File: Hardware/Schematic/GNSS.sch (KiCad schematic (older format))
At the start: 1 part

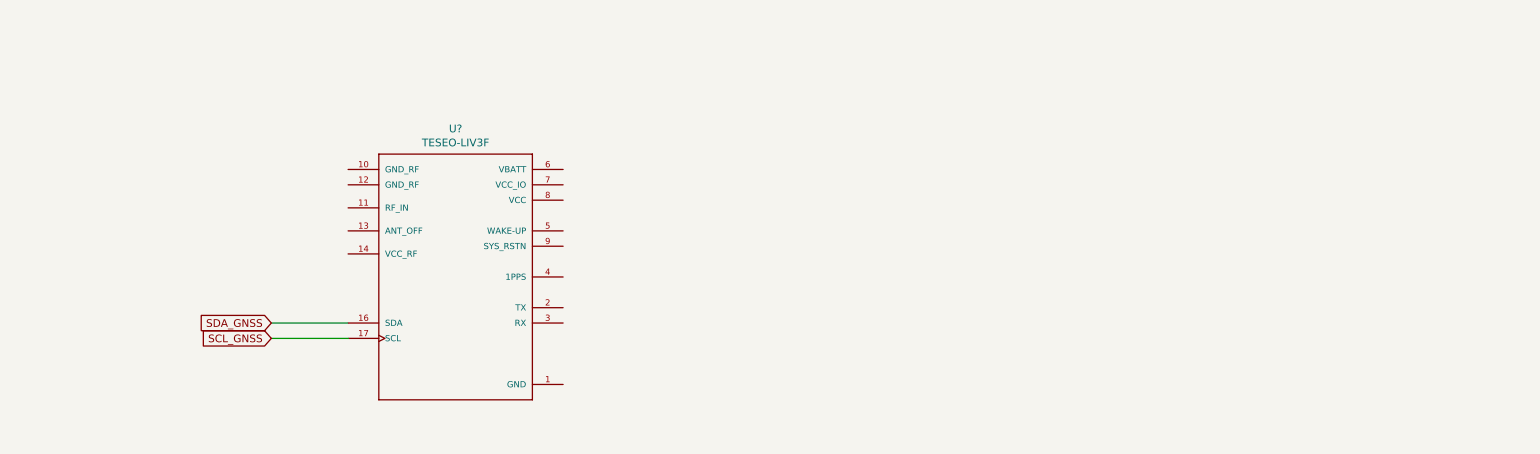
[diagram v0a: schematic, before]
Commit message: Add files via upload
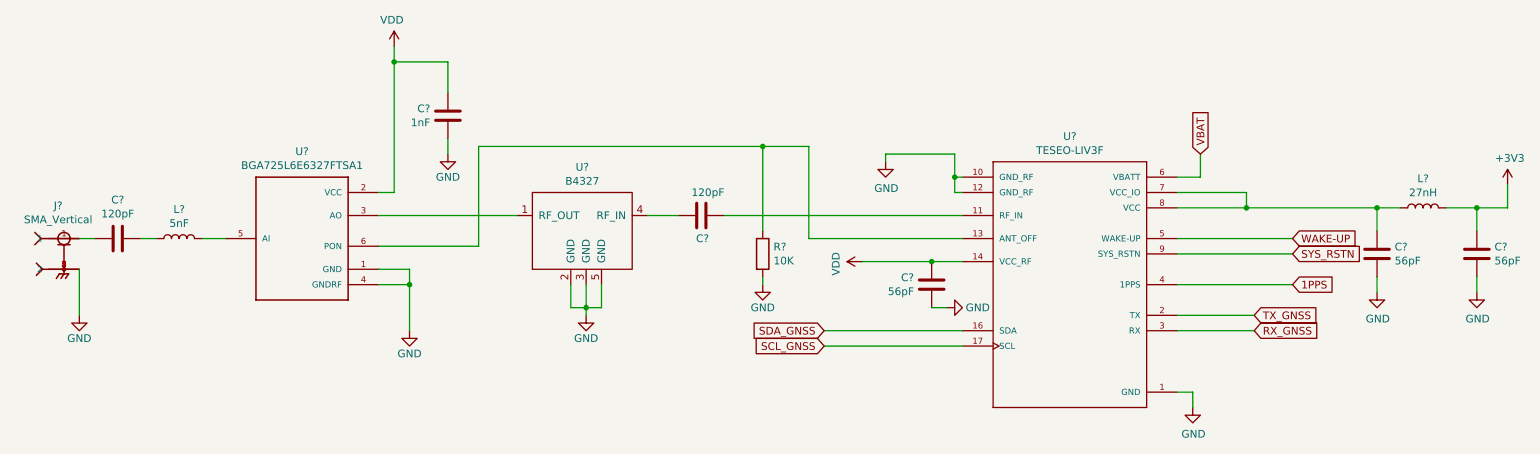
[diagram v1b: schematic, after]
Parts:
- added C? (x3): 56pF, symbol Device:C
- added C?: 1nF, symbol Device:C
- added C? (x2): 120pF, symbol Device:C
- added J?: SMA_Vertical, ASSETS:SMA_Vertical, symbol Regular_Use:SMA_Vertical
- added L?: 27nH, symbol Device:L
- added L?: 5nF, symbol Device:L
- added R?: 10K, symbol Device:R
- added U?: BGA725L6E6327FTSA1, ASSETS:BGA725L6E6327, symbol Regular_Use:BGA725L6E6327FTSA1
- added U?: B4327, ASSETS:B4327, symbol Regular_Use:B4327
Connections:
- net GND: now reaches U?.1 (GND)
- net GND: now also U?.10 (GND_RF), U?.12 (GND_RF), C?.2, C?.2, C?.2, C?.2, J?.2, J?.3 (2), J?.4 (2), J?.5 (2), R?.2, U?.1 (GND), U?.2 (GND), U?.3 (GND), U?.4 (GNDRF), U?.5 (GND)
- net at U?.11 (RF_IN): now also C?.2
- net at U?.13 (ANT_OFF): now also R?.1, U?.6 (PON)
- net VDD: now reaches U?.14 (VCC_RF)
- net VDD: now also C?.1, C?.1, U?.2 (VCC)
- net TX_GNSS: now reaches U?.2 (TX)
- net RX_GNSS: now reaches U?.3 (RX)
- net 1PPS: now reaches U?.4 (1PPS)
- net WAKE-UP: now reaches U?.5 (WAKE-UP)
- net VBAT: now reaches U?.6 (VBATT)
- net at U?.7 (VCC_IO): now also U?.8 (VCC), C?.1, L?.1
- net SYS_RSTN: now reaches U?.9 (SYS_RSTN)
- new net: C?.1, U?.4 (RF_IN)
- new net: C?.1, L?.1
- new net: L?.2, U?.5 (AI)
- new net: C?.2, J?.1
- new net: U?.1 (RF_OUT), U?.3 (AO)
- new net +3V3: C?.1, L?.2
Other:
- moved on the sheet: U?
